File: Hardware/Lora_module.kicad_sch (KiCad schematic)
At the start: 5 parts, among them U12 LORA1276-C1-915MHZ

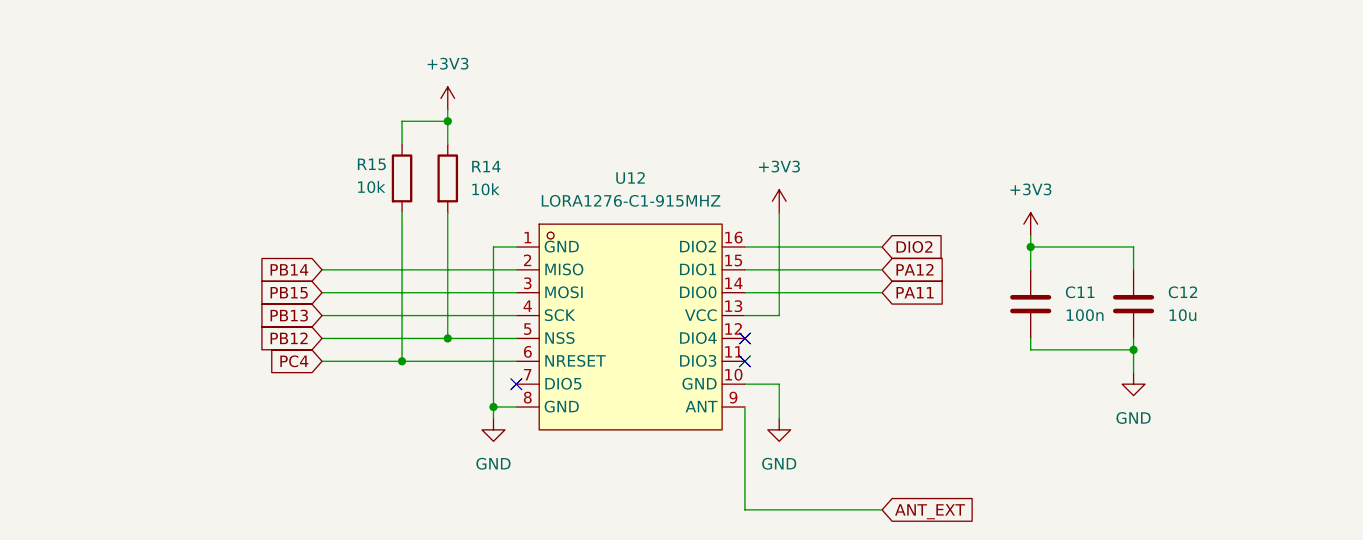
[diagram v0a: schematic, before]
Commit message: design sensores pronto
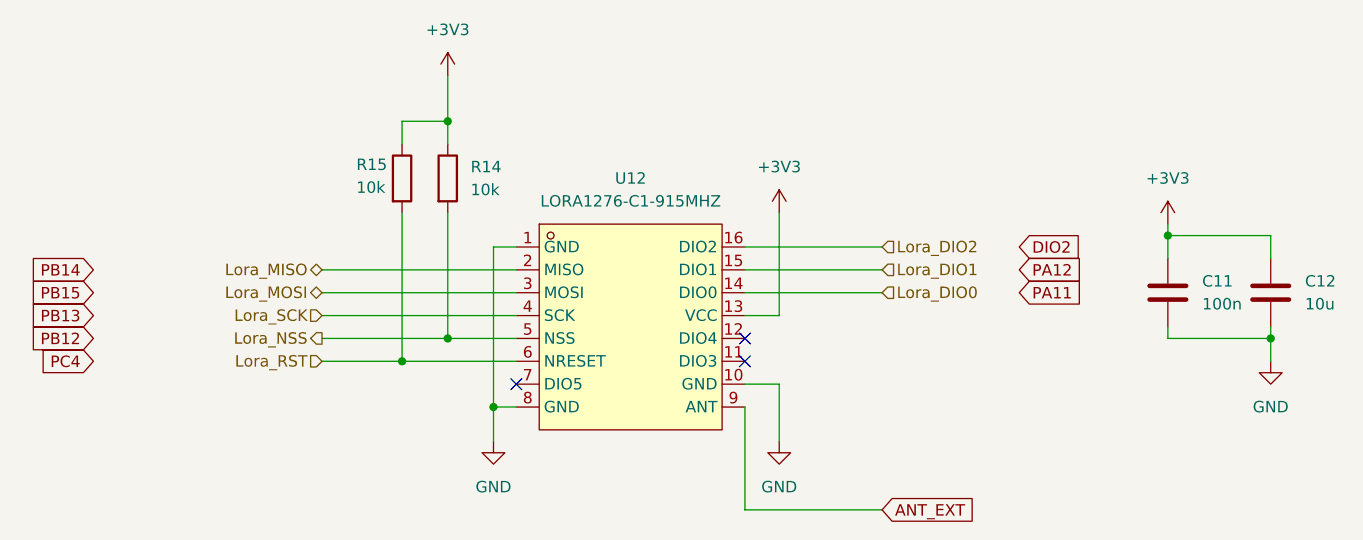
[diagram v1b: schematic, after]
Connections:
- net DIO2: no longer U12.16 (DIO2)
- net PA11: no longer U12.14 (DIO0)
- net PA12: no longer U12.15 (DIO1)
- net PB12: no longer R14.2, U12.5 (NSS)
- net PB13: no longer U12.4 (SCK)
- net PB14: no longer U12.2 (MISO)
- net PB15: no longer U12.3 (MOSI)
- net PC4: no longer R15.2, U12.6 (NRESET)
- new net Lora_DIO0: U12.14 (DIO0)
- new net Lora_DIO1: U12.15 (DIO1)
- new net Lora_DIO2: U12.16 (DIO2)
- new net Lora_MISO: U12.2 (MISO)
- new net Lora_MOSI: U12.3 (MOSI)
- new net Lora_NSS: R14.2, U12.5 (NSS)
- new net Lora_RST: R15.2, U12.6 (NRESET)
- new net Lora_SCK: U12.4 (SCK)
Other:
- moved on the sheet: C11, C12
